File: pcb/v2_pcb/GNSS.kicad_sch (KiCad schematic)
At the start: 22 parts, among them J900 U.FL / Beitian BT-T076, U900 UM980

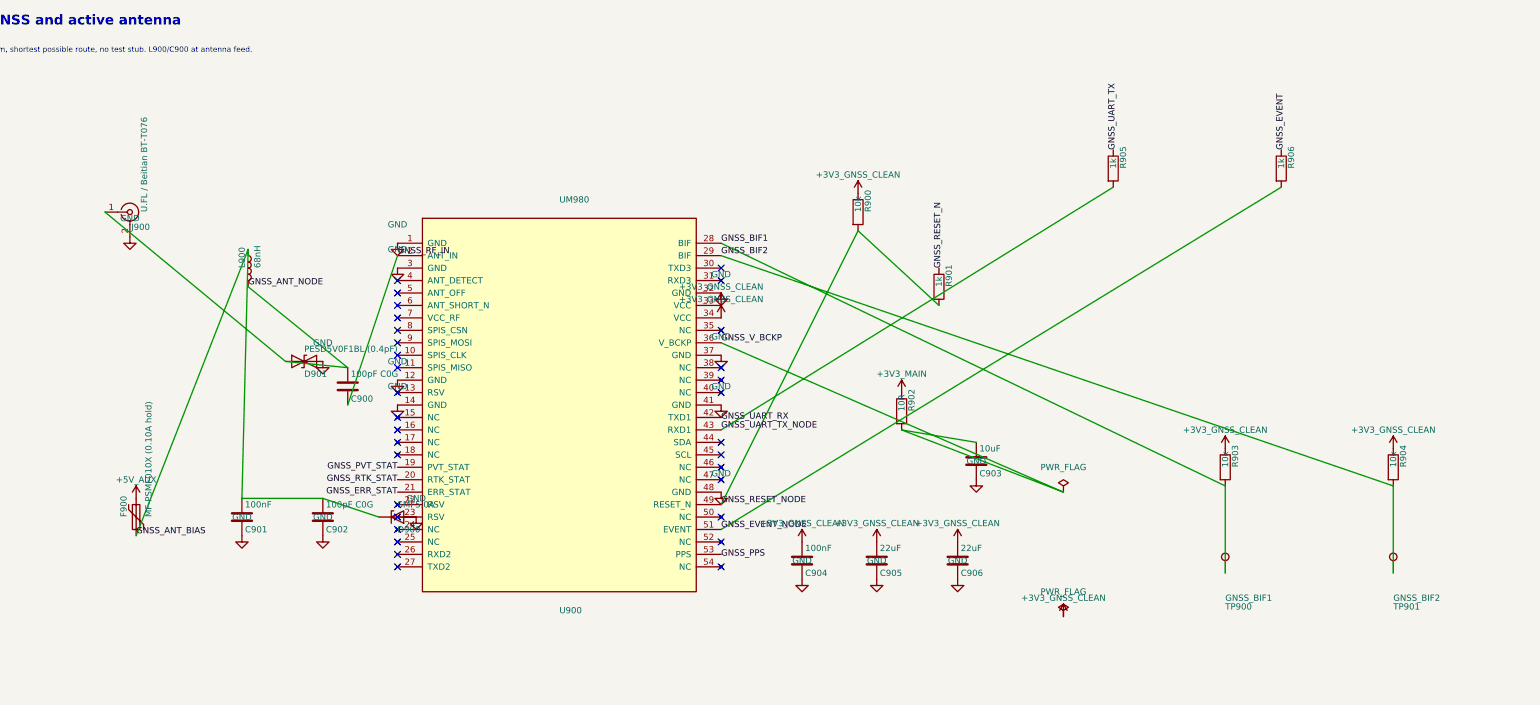
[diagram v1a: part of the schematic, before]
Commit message: clean debug and gnss
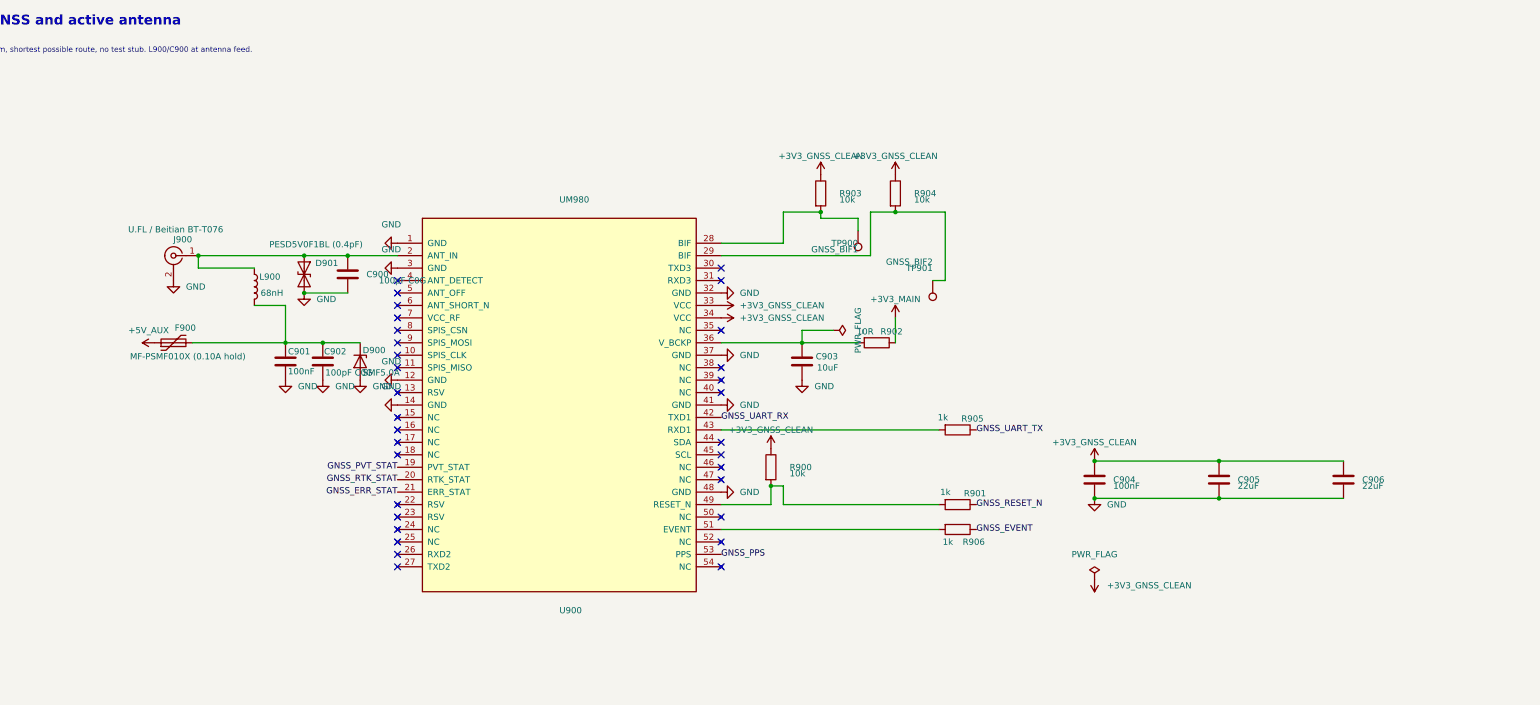
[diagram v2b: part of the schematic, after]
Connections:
- net GND: now also C900.2
- net GNSS_ANT_BIAS: no longer names the net of C901.1, C902.1, D900.1 (K), F900.2
- net GNSS_ANT_BIAS: now also L900.2; no longer L900.1
- net GNSS_ANT_NODE: no longer names the net of C900.1, D901.1 (A1), J900.1 (In)
- net GNSS_ANT_NODE: now also L900.1, U900.2 (ANT_IN); no longer L900.2
- net GNSS_BIF1: no longer names the net of R903.2, TP900.1, U900.28 (BIF)
- net GNSS_BIF2: no longer names the net of R904.2, TP901.1, U900.29 (BIF)
- net GNSS_EVENT_NODE: no longer names the net of R906.2, U900.51 (EVENT)
- net GNSS_RESET_NODE: no longer names the net of R900.2, R901.2, U900.49 (RESET_N)
- removed net GNSS_RF_IN: C900.2, U900.2 (ANT_IN)
- net GNSS_UART_TX_NODE: no longer names the net of R905.2, U900.43 (RXD1)
- net GNSS_V_BCKP: no longer names the net of C903.1, R902.2, U900.36 (V_BCKP)
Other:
- moved on the sheet: C900, C901, C902, C903, C904, C905, C906, D900, D901, F900, J900, L900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
